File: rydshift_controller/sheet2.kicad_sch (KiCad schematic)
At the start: 43 parts, among them IC1 PMA3-43-1W+, IC2 PMA3-43-1W+, IC3 PMA3-43-1W+, IC4 PMA3-43-1W+, IC5 SYPS-2-22HP+, IC6 SYPS-2-22HP+, IC7 ADL5513ACPZ-R7

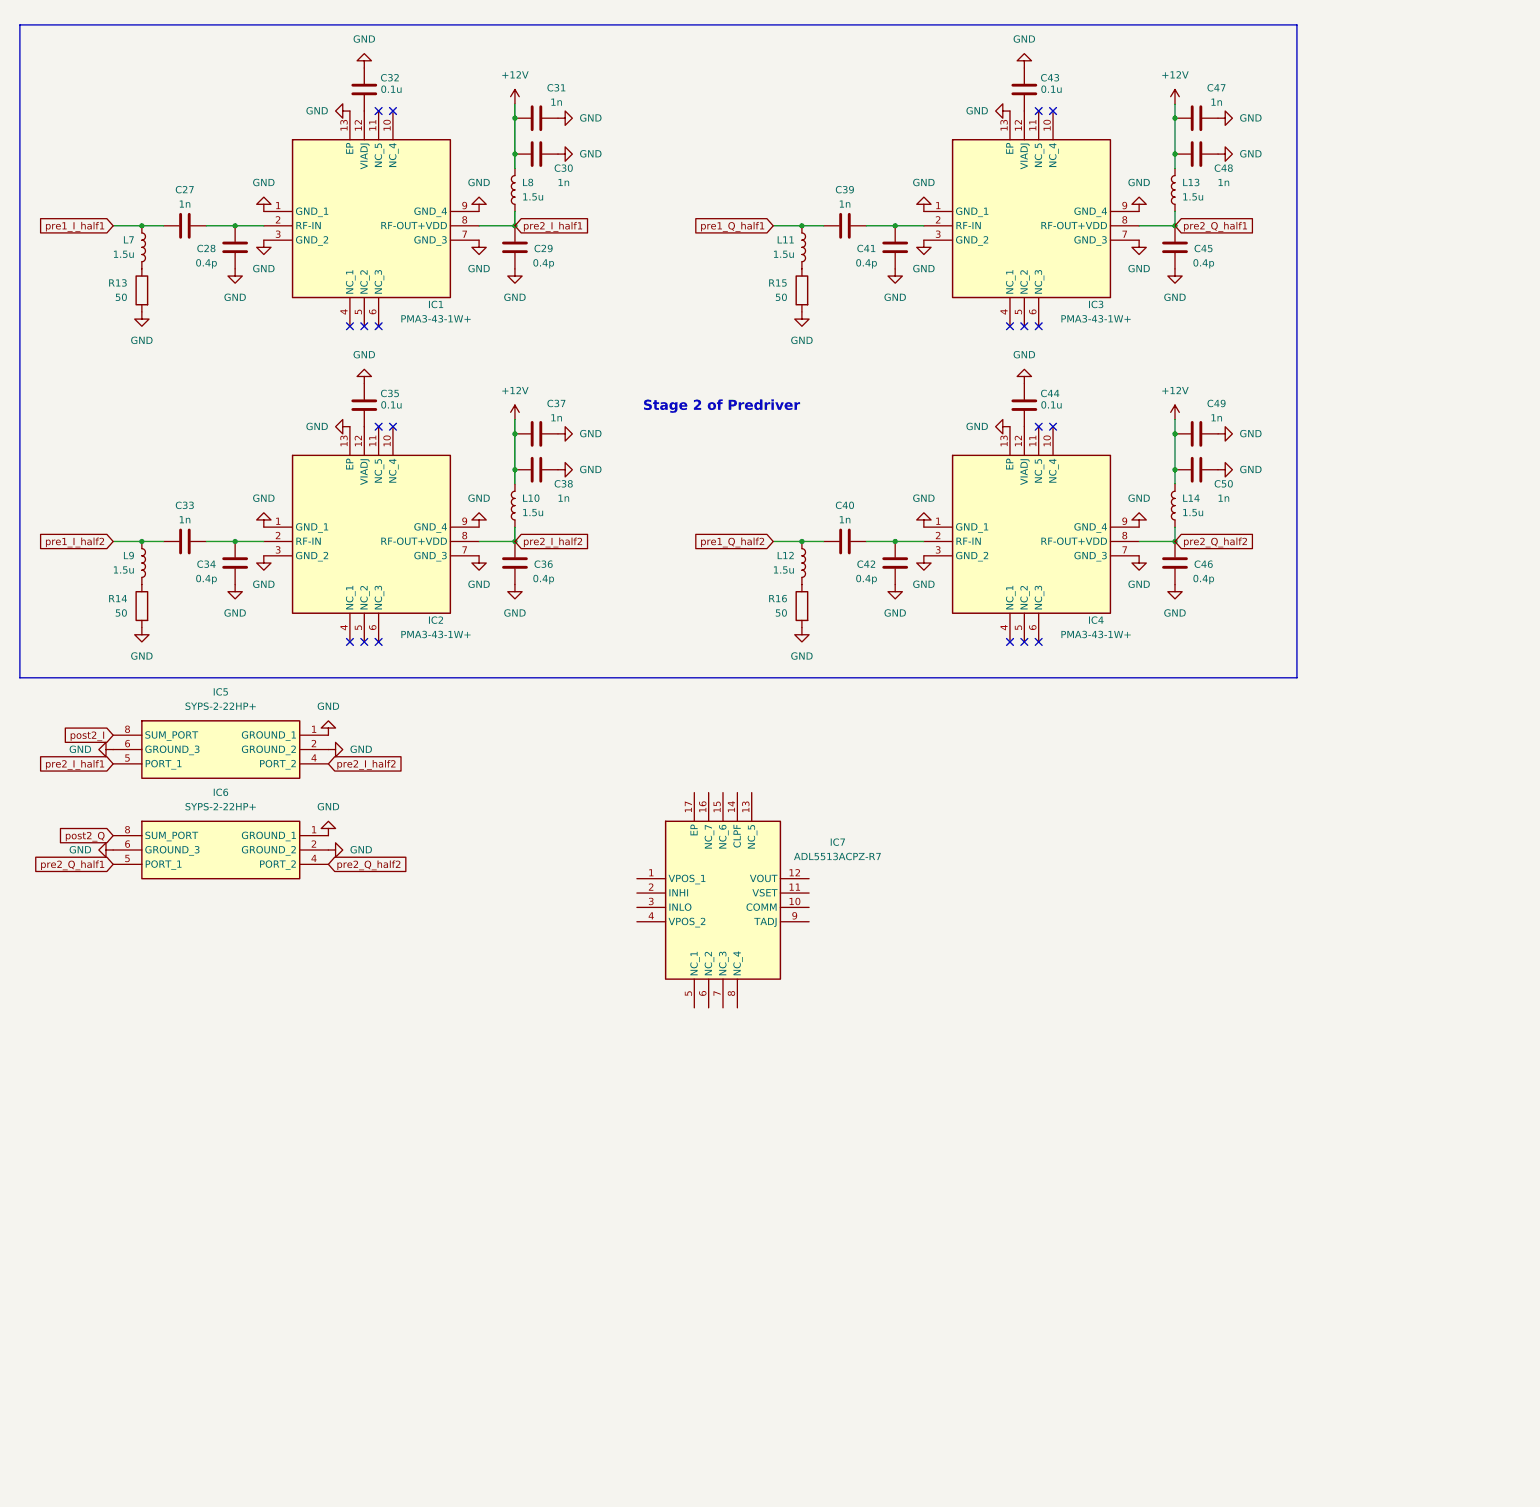
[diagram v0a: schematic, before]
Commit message: added feedback to controller
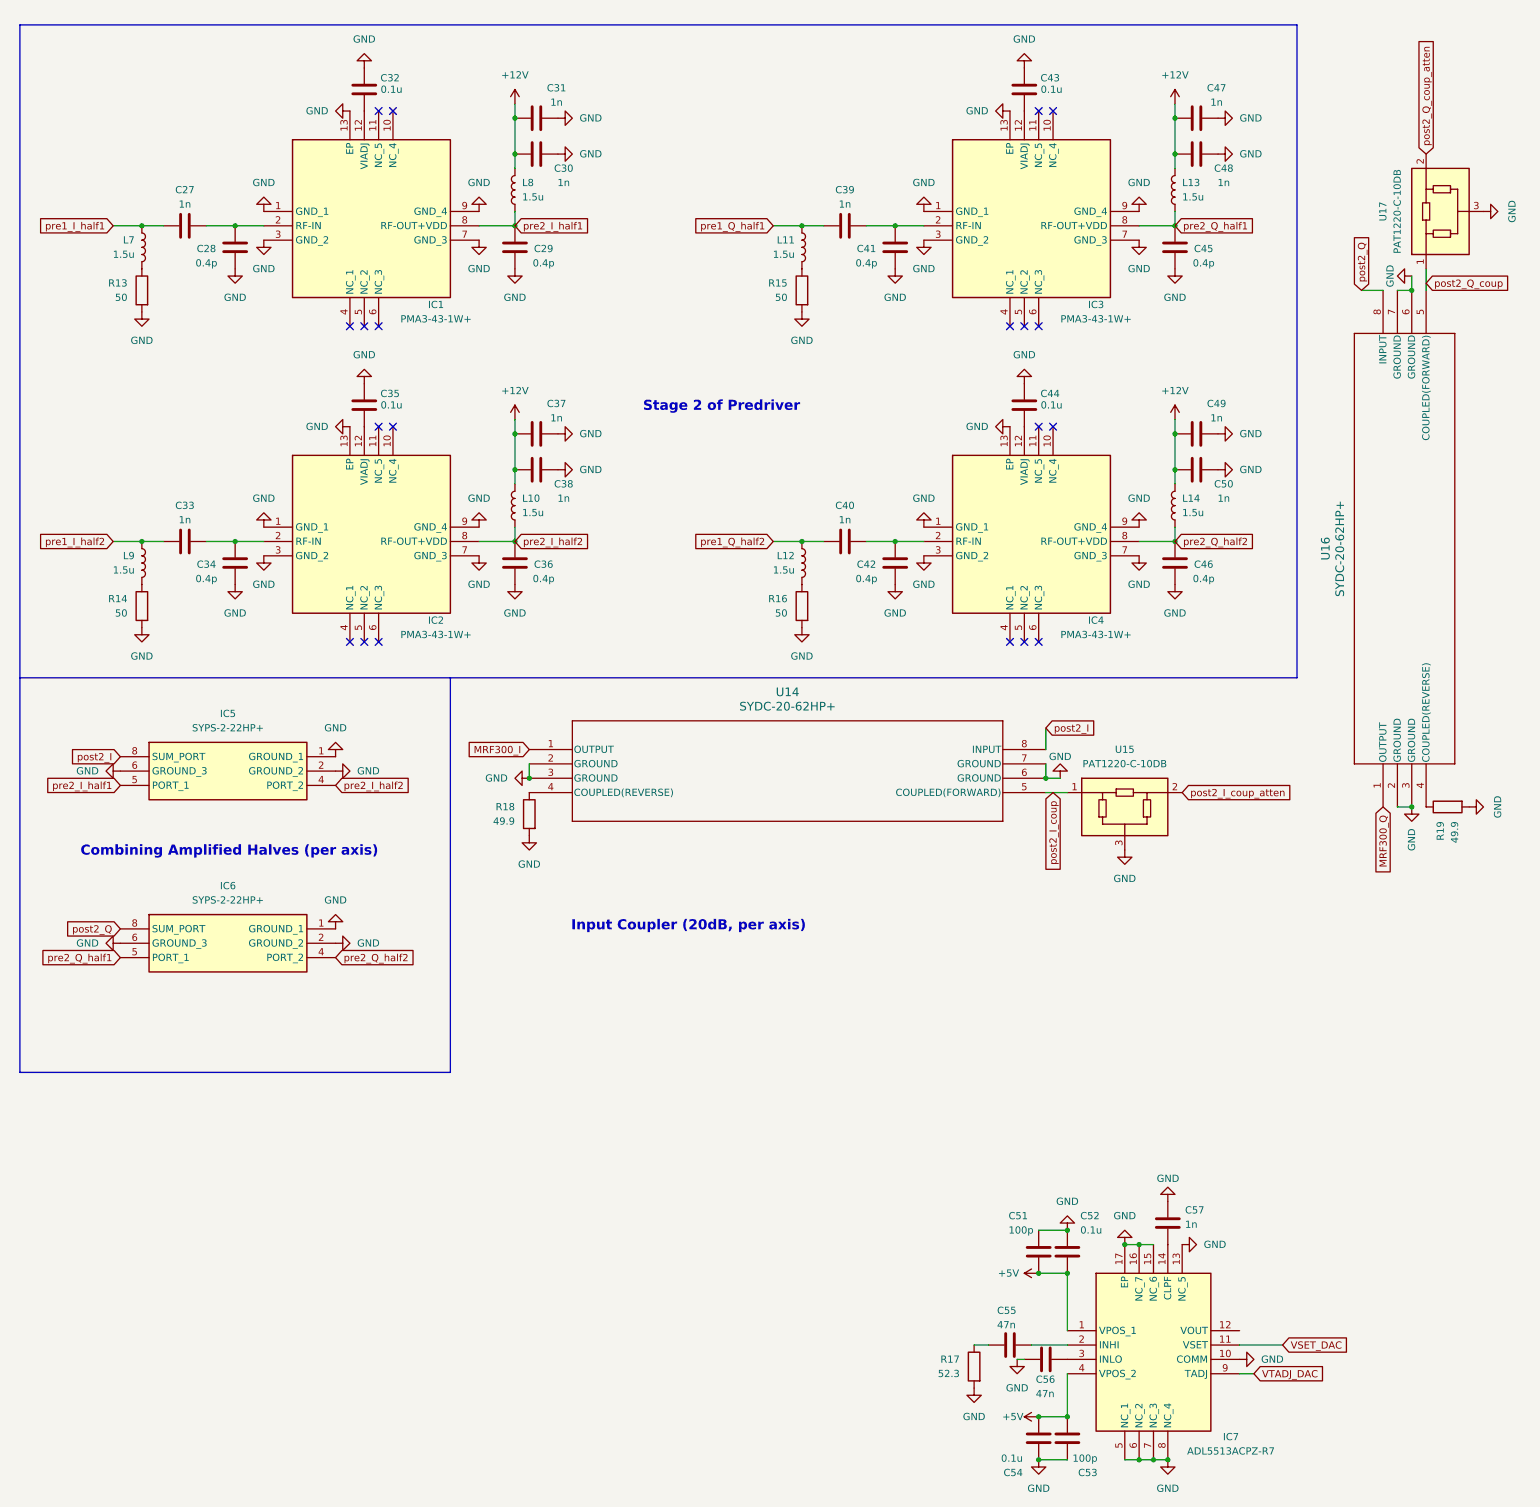
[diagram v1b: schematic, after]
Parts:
- added C51, C53: 100p, symbol Device:C
- added C52, C54: 0.1u, symbol Device:C
- added C55, C56: 47n, symbol Device:C
- added C57: 1n, symbol Device:C
- added R17: 52.3, symbol Device:R
- added R18, R19: 49.9, symbol Device:R
- added U14, U16: SYDC-20-62HP+, AH202-1_MNC, symbol SYDC-20-22HP+:SYDC-20-62HP+
- added U15, U17: PAT1220-C-10DB, RF_Converter:RF_Attenuator_Susumu_PAT1220, symbol RF:PAT1220-C-10DB
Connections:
- net GND: now also IC7.10 (COMM), IC7.13 (NC_5), IC7.15 (NC_6), IC7.16 (NC_7), IC7.17 (EP), IC7.5 (NC_1), IC7.6 (NC_2), IC7.7 (NC_3), IC7.8 (NC_4), C51.1, C52.2, C53.1, C54.2, C56.1, C57.2, R17.2, R18.2, R19.2, U14.2 (GROUND), U14.3 (GROUND), U14.6 (GROUND), U14.7 (GROUND), U15.3, U16.2 (GROUND), U16.3 (GROUND), U16.6 (GROUND), U16.7 (GROUND), U17.3
- net post2_I: now also U14.8 (INPUT)
- net post2_Q: now also U16.8 (INPUT)
- net +5V: now reaches IC7.1 (VPOS_1)
- net +5V: now also IC7.4 (VPOS_2), C51.2, C52.1, C53.2, C54.1
- net VSET_DAC: now reaches IC7.11 (VSET)
- net at IC7.14 (CLPF): now also C57.1
- net at IC7.2 (INHI): now also C55.2
- net at IC7.3 (INLO): now also C56.2
- net VTADJ_DAC: now reaches IC7.9 (TADJ)
- new net: C55.1, R17.1
- new net: R19.1, U16.4 (COUPLED(REVERSE))
- new net: R18.1, U14.4 (COUPLED(REVERSE))
- new net MRF300_I: U14.1 (OUTPUT)
- new net MRF300_Q: U16.1 (OUTPUT)
- new net post2_I_coup: U14.5 (COUPLED(FORWARD)), U15.1
- new net post2_I_coup_atten: U15.2
- new net post2_Q_coup: U16.5 (COUPLED(FORWARD)), U17.1
- new net post2_Q_coup_atten: U17.2
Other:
- note added: "Combining Amplified Halves (per axis)"
- note added: "Input Coupler (20dB, per axis)"
- moved on the sheet: IC5, IC6, IC7
